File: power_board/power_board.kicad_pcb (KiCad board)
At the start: 2 copper layers, 73 x 109.5 mm, 26 parts, among them J1 From Trfo Output, J2 IN 12V AC, J3 OUT 230V AC, J4 IN 230V AC, J5 To Power Ampli Power IN, J6 OUT 5V CC, J7 From Ampli Output, J8 To Speakers, J9 OUT 12V CC, K1 SANYOU_SRD_Form_C, K2 SANYOU_SRD_Form_C, Q1 BC171, Q2 BD235, U1 LM7812_TO220

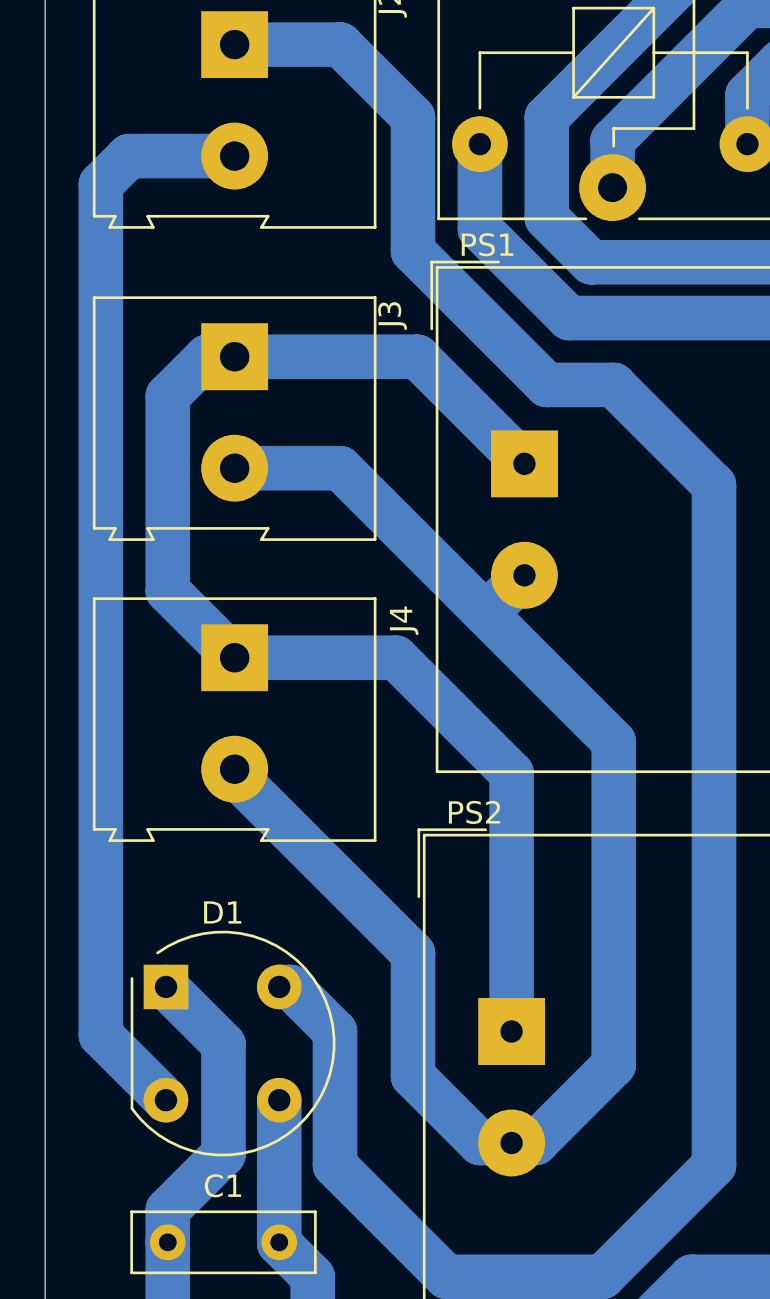
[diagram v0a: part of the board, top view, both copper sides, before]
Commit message: Power board.
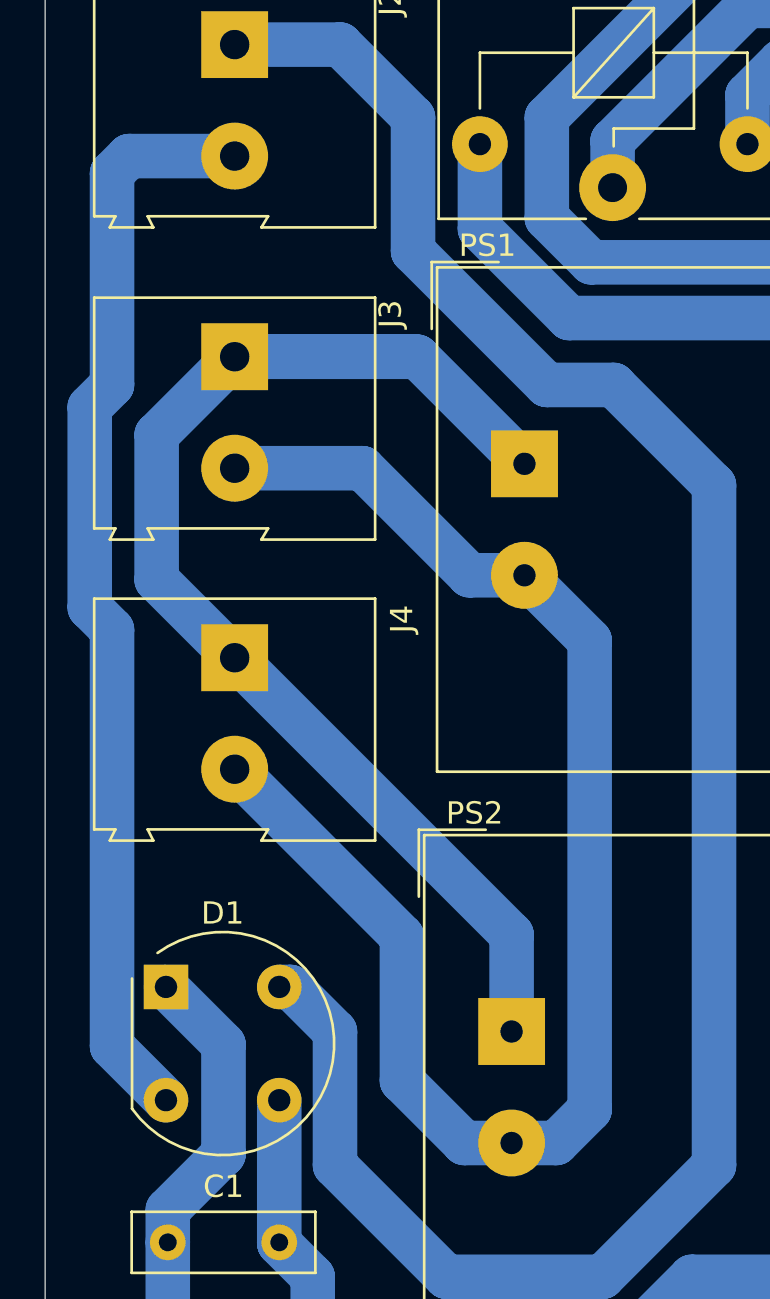
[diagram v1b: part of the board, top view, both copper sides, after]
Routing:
- net 230VAC: track 57.8 -> 61.4 mm
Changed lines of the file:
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@@
 		)
 		(property "Value" "IN 230V AC"
-			(at 2.78 7.75 90)
+			(at 2.78 7 90)
 			(layer "F.Fab")
 			(effects
@@
 		)
 		(property "Value" "IN 12V AC"
-			(at 2.78 7.75 90)
+			(at 2.78 7 90)
 			(layer "F.Fab")
 			(effects
@@
 		)
 		(property "Value" "OUT 230V AC"
-			(at 2.78 7.75 90)
+			(at 2.78 7 90)
 			(layer "F.Fab")
 			(effects
@@
 	)
 	(segment
-		(start 36 103.16)
-		(end 36 65)
+		(start 35.499 83.978055)
+		(end 35.499 74.991946)
+		(width 2)
+		(layer "B.Cu")
+		(net 6)
+	)
+	(segment
+		(start 36.5 84.979055)
+		(end 35.499 83.978055)
 		(width 2)
 		(layer "B.Cu")
@@
 	)
 	(segment
-		(start 36 65)
+		(start 38.92 106.08)
+		(end 36.5 103.66)
+		(width 2)
+		(layer "B.Cu")
+		(net 6)
+	)
+	(segment
+		(start 36.5 64.5)
 		(end 37.265 63.735)
 		(width 2)
@@
 	)
 	(segment
-		(start 38.92 106.08)
-		(end 36 103.16)
+		(start 36.5 73.990945)
+		(end 36.5 64.5)
+		(width 2)
+		(layer "B.Cu")
+		(net 6)
+	)
+	(segment
+		(start 36.5 103.66)
+		(end 36.5 84.979055)
+		(width 2)
+		(layer "B.Cu")
+		(net 6)
+	)
+	(segment
+		(start 35.499 74.991946)
+		(end 36.5 73.990945)
 		(width 2)
 		(layer "B.Cu")
@@
 	)
 	(segment
-		(start 42 91.5)
-		(end 50 99.5)
+		(start 49.501 105.20232)
+		(end 49.501 98.736)
 		(width 2)
 		(layer "B.Cu")
@@
 	)
 	(segment
-		(start 50 99.5)
-		(end 50 105)
+		(start 49.501 98.736)
+		(end 42 91.235)
 		(width 2)
 		(layer "B.Cu")
@@
 	)
 	(segment
-		(start 53 108)
-		(end 54.42 108)
+		(start 47.735 77.735)
+		(end 52.5375 82.5375)
 		(width 2)
 		(layer "B.Cu")
@@
 	)
 	(segment
-		(start 50 105)
-		(end 53 108)
+		(start 52.29868 108)
+		(end 49.501 105.20232)
 		(width 2)
 		(layer "B.Cu")
@@
 	)
 	(segment
-		(start 53.285 84.25)
-		(end 53.25 84.25)
+		(start 52.5375 82.5375)
+		(end 54.9975 82.5375)
 		(width 2)
 		(layer "B.Cu")
@@
 	)
 	(segment
-		(start 59 90)
-		(end 53.25 84.25)
+		(start 42 77.735)
+		(end 47.735 77.735)
 		(width 2)
 		(layer "B.Cu")
@@
 	)
 	(segment
-		(start 42 91.235)
-		(end 42 91.5)
+		(start 57.921 85.461)
+		(end 57.921 106.501)
 		(width 2)
 		(layer "B.Cu")
@@
 	)
 	(segment
-		(start 55.5 108)
-		(end 59 104.5)
+		(start 57.921 106.501)
+		(end 56.422 108)
 		(width 2)
 		(layer "B.Cu")
@@
 	)
 	(segment
-		(start 54.42 108)
-		(end 55.5 108)
-		(width 2)
-		(layer "B.Cu")
-		(net 25)
-	)
-	(segment
-		(start 54.9975 82.5375)
-		(end 53.285 84.25)
-		(width 2)
-		(layer "B.Cu")
-		(net 25)
-	)
-	(segment
-		(start 53.25 84.25)
-		(end 46.735 77.735)
+		(start 56.422 108)
+		(end 54.42 108)
 		(width 2)
 		(layer "B.Cu")
@@
 	)
 	(segment
-		(start 46.735 77.735)
-		(end 42 77.735)
+		(start 54.42 108)
+		(end 52.29868 108)
 		(width 2)
 		(layer "B.Cu")
@@
 	)
 	(segment
-		(start 59 104.5)
-		(end 59 90)
+		(start 54.9975 82.5375)
+		(end 57.921 85.461)
 		(width 2)
 		(layer "B.Cu")
@@
 	)
 	(segment
-		(start 54.42 91.42)
-		(end 49.235 86.235)
-		(width 2)
-		(layer "B.Cu")
-		(net 26)
-	)
-	(segment
-		(start 54.42 103)
-		(end 54.42 91.42)
+		(start 42 72.735)
+		(end 50.146162 72.735)
 		(width 2)
 		(layer "B.Cu")
@@
 	)
 	(segment
-		(start 39 74.5)
-		(end 39 83.235)
+		(start 38.5 82.735)
+		(end 42 86.235)
 		(width 2)
 		(layer "B.Cu")
@@
 	(segment
 		(start 42 72.735)
-		(end 40.765 72.735)
+		(end 50.195 72.735)
 		(width 2)
 		(layer "B.Cu")
@@
 	)
 	(segment
-		(start 49.235 86.235)
-		(end 42 86.235)
+		(start 42 72.735)
+		(end 38.5 76.235)
 		(width 2)
 		(layer "B.Cu")
@@
 	)
 	(segment
-		(start 39 83.235)
-		(end 42 86.235)
+		(start 38.5 76.235)
+		(end 38.5 82.735)
 		(width 2)
 		(layer "B.Cu")
@@
 	)
 	(segment
-		(start 40.765 72.735)
-		(end 39 74.5)
+		(start 42 86.235)
+		(end 54.42 98.655)
 		(width 2)
 		(layer "B.Cu")
@@
 	)
 	(segment
-		(start 42 72.735)
-		(end 50.195 72.735)
+		(start 54.42 98.655)
+		(end 54.42 103)
 		(width 2)
 		(layer "B.Cu")
